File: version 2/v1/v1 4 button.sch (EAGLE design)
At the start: 38 parts, among them IC5 AMS1117-3.3V, X1 0446200002

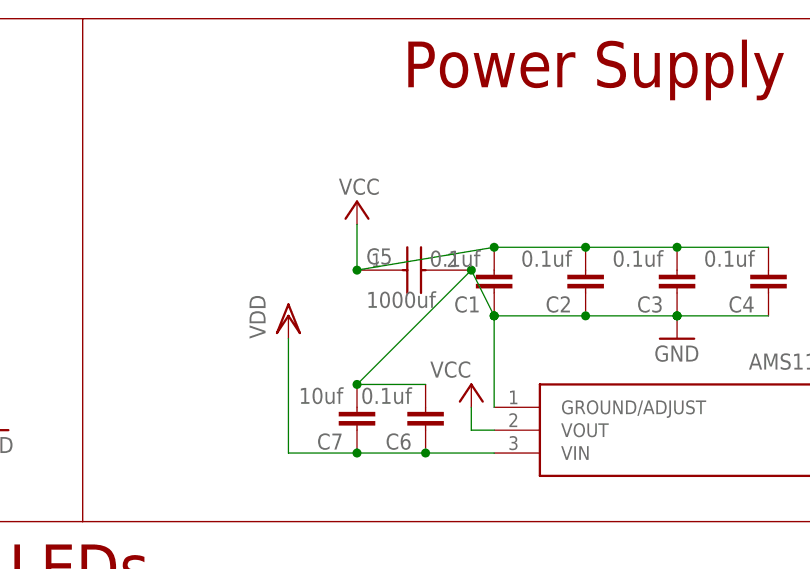
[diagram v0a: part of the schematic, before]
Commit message: Add files via upload
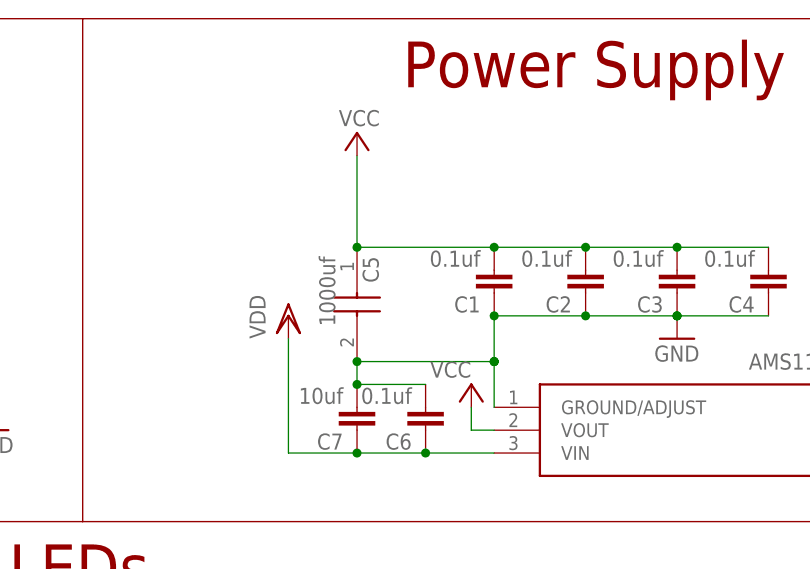
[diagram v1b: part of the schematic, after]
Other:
- moved on the sheet: C5
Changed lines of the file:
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@@
 <attribute name="VALUE" x="196.596" y="121.539" size="1.778" layer="96" rot="R180"/>
 </instance>
-<instance part="C5" gate="G$1" x="152.4" y="119.38" smashed="yes">
-<attribute name="NAME" x="153.416" y="120.015" size="1.778" layer="95"/>
-<attribute name="VALUE" x="153.416" y="115.189" size="1.778" layer="96"/>
+<instance part="C5" gate="G$1" x="152.4" y="121.92" smashed="yes" rot="R270">
+<attribute name="NAME" x="153.035" y="120.904" size="1.778" layer="95" rot="R270"/>
+<attribute name="VALUE" x="148.209" y="120.904" size="1.778" layer="96" rot="R270"/>
 </instance>
 <instance part="IC5" gate="G$1" x="167.64" y="104.14" smashed="yes">
@@
 <attribute name="VALUE" x="17.78" y="132.08" size="1.778" layer="96" rot="R180"/>
 </instance>
-<instance part="P+1" gate="VCC" x="152.4" y="127" smashed="yes">
-<attribute name="VALUE" x="154.94" y="129.54" size="1.778" layer="96" rot="R180"/>
+<instance part="P+1" gate="VCC" x="152.4" y="134.62" smashed="yes">
+<attribute name="VALUE" x="154.94" y="137.16" size="1.778" layer="96" rot="R180"/>
 </instance>
 <instance part="P+2" gate="VCC" x="165.1" y="106.68" smashed="yes">
@@
 <pinref part="C5" gate="G$1" pin="+"/>
 <pinref part="P+1" gate="VCC" pin="VCC"/>
-<wire x1="152.4" y1="119.38" x2="152.4" y2="124.46" width="0.1524" layer="91"/>
+<wire x1="152.4" y1="121.92" x2="152.4" y2="132.08" width="0.1524" layer="91"/>
 <pinref part="C1" gate="G$1" pin="2"/>
-<wire x1="152.4" y1="119.38" x2="167.64" y2="121.92" width="0.1524" layer="91"/>
-<junction x="152.4" y="119.38"/>
+<wire x1="152.4" y1="121.92" x2="167.64" y2="121.92" width="0.1524" layer="91"/>
+<junction x="152.4" y="121.92"/>
 <pinref part="C2" gate="G$1" pin="2"/>
 <wire x1="167.64" y1="121.92" x2="177.8" y2="121.92" width="0.1524" layer="91"/>
@@
 <net name="GND" class="0">
 <segment>
-<pinref part="C7" gate="G$1" pin="2"/>
-<pinref part="C6" gate="G$1" pin="2"/>
 <pinref part="IC5" gate="G$1" pin="GROUND/ADJUST"/>
-<wire x1="152.4" y1="106.68" x2="160.02" y2="106.68" width="0.1524" layer="91"/>
-<wire x1="167.64" y1="104.14" x2="167.64" y2="114.3" width="0.1524" layer="91"/>
+<wire x1="167.64" y1="104.14" x2="167.64" y2="109.22" width="0.1524" layer="91"/>
 <pinref part="C1" gate="G$1" pin="1"/>
-<pinref part="C5" gate="G$1" pin="-"/>
-<wire x1="167.64" y1="114.3" x2="165.1" y2="119.38" width="0.1524" layer="91"/>
 <junction x="167.64" y="114.3"/>
-<wire x1="152.4" y1="106.68" x2="165.1" y2="119.38" width="0.1524" layer="91"/>
-<junction x="152.4" y="106.68"/>
-<junction x="165.1" y="119.38"/>
 <pinref part="C2" gate="G$1" pin="1"/>
+<wire x1="167.64" y1="109.22" x2="167.64" y2="114.3" width="0.1524" layer="91"/>
 <wire x1="167.64" y1="114.3" x2="177.8" y2="114.3" width="0.1524" layer="91"/>
-<junction x="167.64" y="114.3"/>
 <pinref part="C3" gate="G$1" pin="1"/>
 <wire x1="177.8" y1="114.3" x2="187.96" y2="114.3" width="0.1524" layer="91"/>
@@
 <junction x="187.96" y="114.3"/>
 <wire x1="187.96" y1="114.3" x2="198.12" y2="114.3" width="0.1524" layer="91"/>
+<pinref part="C5" gate="G$1" pin="-"/>
+<pinref part="C6" gate="G$1" pin="2"/>
+<pinref part="C7" gate="G$1" pin="2"/>
+<wire x1="152.4" y1="106.68" x2="160.02" y2="106.68" width="0.1524" layer="91"/>
+<wire x1="152.4" y1="106.68" x2="152.4" y2="109.22" width="0.1524" layer="91"/>
+<junction x="152.4" y="106.68"/>
+<wire x1="152.4" y1="109.22" x2="167.64" y2="109.22" width="0.1524" layer="91"/>
+<junction x="152.4" y="109.22"/>
+<junction x="167.64" y="109.22"/>
 </segment>
 <segment>
@@
 </segment>
 </net>
+<net name="N$19" class="0">
+<segment>
+<junction x="167.64" y="109.22"/>
+</segment>
+</net>
